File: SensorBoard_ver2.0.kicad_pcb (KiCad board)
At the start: 2 copper layers, 93.1 x 58 mm, 59 parts, among them IC1 MIC5504-3.3YM5-T5, J1 CANConn, J10 USB_C, J13 Abso, J14 Abso, J15 STLink, J16 Abso, J18 Abso, J19 Abso, J2 CANConn, J20 Enc5, J3 Enc1, J4 Enc2, J5 Enc3, J6 Enc4, SW1 CAN_Terminal, SW2 IDSetSW, SW3 Reset, SW4 IDSetSW, SW5 Terminal, U1 L7805, U2 ATA6561, U4 STM32F303K8Tx, U5 MAX3485, Y1 Crystal

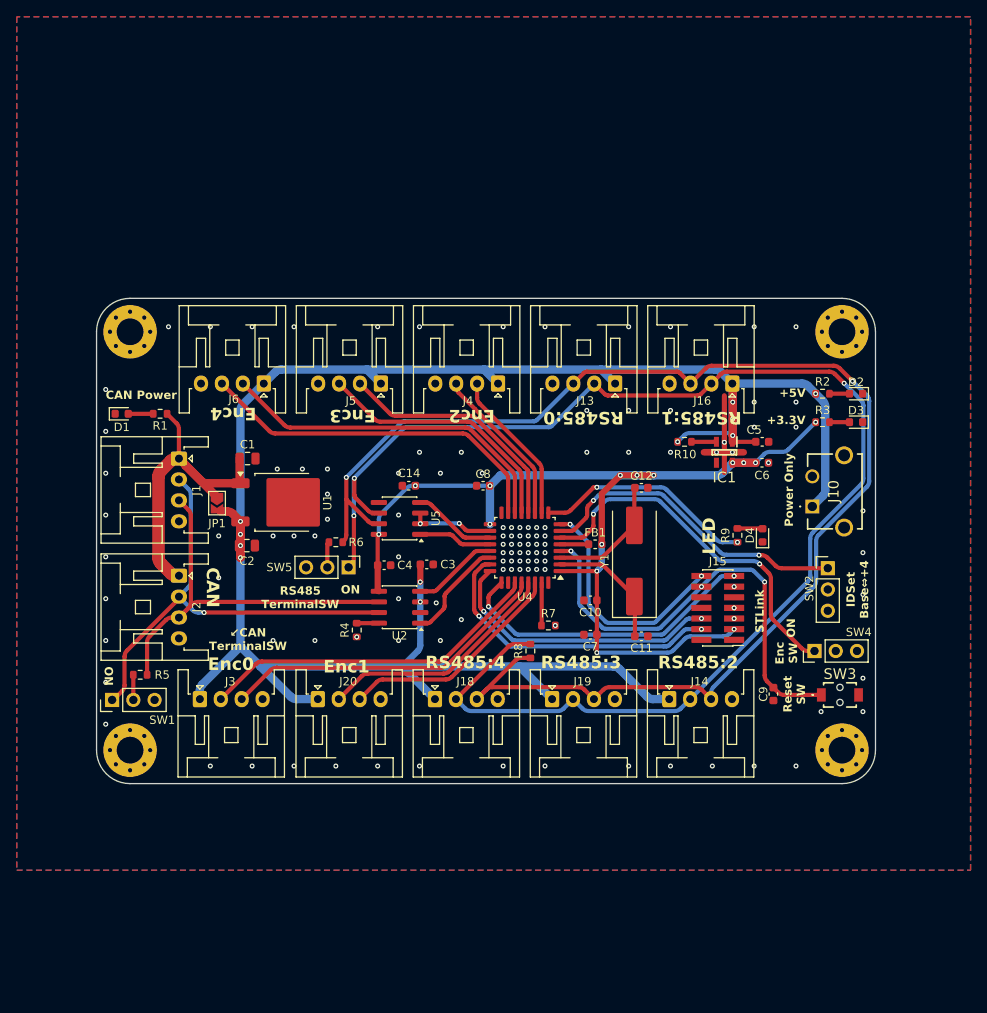
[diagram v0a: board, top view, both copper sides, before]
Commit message: 大改造したあと　ver01
特になし、アップロードしたファイル間違えてるかもしれないくらい？
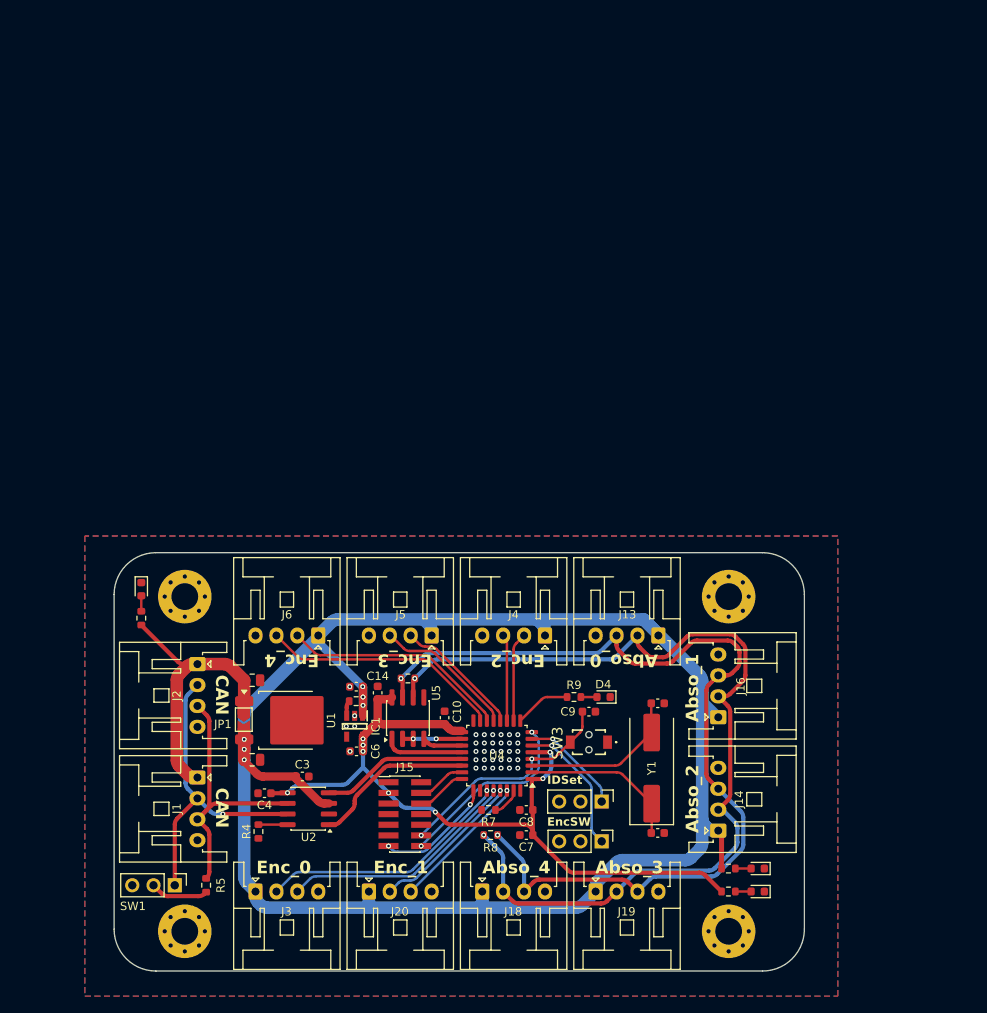
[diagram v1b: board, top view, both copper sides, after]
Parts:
- removed FB1: FerriteBead, Inductor_SMD:L_0603_1608Metric
- removed H5: Hamada, MySilcscreen:Hamada
- removed J10: USB_C, MyUSB_C:PowerOnlyUSB_C
- removed SW5: Terminal, Connector_PinHeader_2.54mm:PinHeader_1x03_P2.54mm_Vertical
- moved H4 84.7 mm to (67.0, 102.2)
- moved H3 78.2 mm to (131.9, 102.2)
- moved C6 59.5 mm to (87.5, 120.7), turned to 180 degrees
- moved D2 58.0 mm to (135.4, 134.8)
- moved R2 57.9 mm to (131.9, 134.8)
- moved D3 57.3 mm to (135.4, 137.5)
- moved R3 57.2 mm to (131.9, 137.5)
- moved C5 56.7 mm to (87.4, 113.0), turned to 180 degrees
- moved IC1 55.0 mm to (87.2, 117.7)
- moved R10 50.0 mm to (87.4, 114.7), turned to 180 degrees
- moved J15 44.8 mm to (93.2, 128.2), turned to 0 degrees
- moved J16 39.9 mm to (130.7, 116.7), turned to 90 degrees
- moved C8 39.1 mm to (107.8, 127.7)
- moved SW2 38.8 mm to (116.8, 126.7), turned to -90 degrees
- moved J1 38.2 mm to (68.5, 123.9)
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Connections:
- R6 pad 1: Net-(SW5-B) -> /RS485_B
- R6 pad 2: /RS485_B -> /RS485_A
- SW3 pad 1: /NRST -> GND
- SW3 pad 2: GND -> /NRST
- U4 pad 5: +3.3VA -> +3.3V
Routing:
- net /RS485_A: track 171.3 -> 113.9 mm, vias 3 -> 2
- net /RS485_B: track 165.8 -> 113.5 mm
- net +5V: track 252.6 -> 214.3 mm, vias 11 -> 6
- net /SWDIO: track 36.4 -> 5.80 mm, vias 2 -> 0
- net /SWCLK: track 33.9 -> 5.99 mm, vias 2 -> 0
- net /EncSW: track 43.5 -> 16.2 mm, vias 2 -> 1
- net /NRST: track 53.9 -> 27.3 mm, vias 3 -> 2
- net /IDSet: track 38.0 -> 12.4 mm, vias 2 -> 1
- net +3.3V: track 121.9 -> 97.6 mm, vias 15 -> 8
- net /VCPRX: track 37.1 -> 14.2 mm
- net /LED: track 26.4 -> 6.71 mm, vias 2 -> 0
- net /CANH: track 55.4 -> 37.6 mm
- net /CANL: track 48.8 -> 33.9 mm
- net /EncA_4: track 41.5 -> 27.2 mm
- net /EncB_4: track 43.1 -> 28.9 mm
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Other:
- board size 93.1 x 58 mm -> 82.5 x 50 mm
- board text added: "Abso_0"
- board text added: "Abso_1"
- board text added: "Abso_2"
- board text added: "Abso_3"
- board text added: "Abso_4"
- board text added: "EncSW"
- board text added: "Enc_0"
- board text added: "Enc_1"
- board text added: "Enc_2"
- board text added: "Enc_3"
- board text added: "Enc_4"
- board text added: "IDSet"
- board text removed: "+3.3V"
- board text removed: "+5V"
- board text removed: "CAN Power"
- board text removed: "Designed by Hama"
- board text removed: "Enc SW"
- board text removed: "Enc0"
- board text removed: "Enc1"
- board text removed: "Enc2"
- board text removed: "Enc3"
- board text removed: "Enc4"
- board text removed: "Firmware:Jaga"
- board text removed: "IDSet Base⇔+4"
- board text removed: "LED"
- board text removed: "ON"
- board text removed: "Power Only"
- board text removed: "RS485 TerminalSW"
- board text removed: "RS485:0"
- board text removed: "RS485:1"
- board text removed: "RS485:2"
- board text removed: "RS485:3"
- board text removed: "RS485:4"
- board text removed: "Reset SW"
- board text removed: "STLink"
- board text removed: "SensorBoard Ver 1.0"
- board text removed: "↙CAN TerminalSW"
